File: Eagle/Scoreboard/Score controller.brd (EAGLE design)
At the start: 69.8 x 40.6 mm, 21 parts, among them IC3 74HC595N, Q1 BC338-40, Q2 BC338-40, Q3 BC338-40, Q4 BC338-40, Q5 BC338-40, Q6 BC338-40, Q7 BC338-40

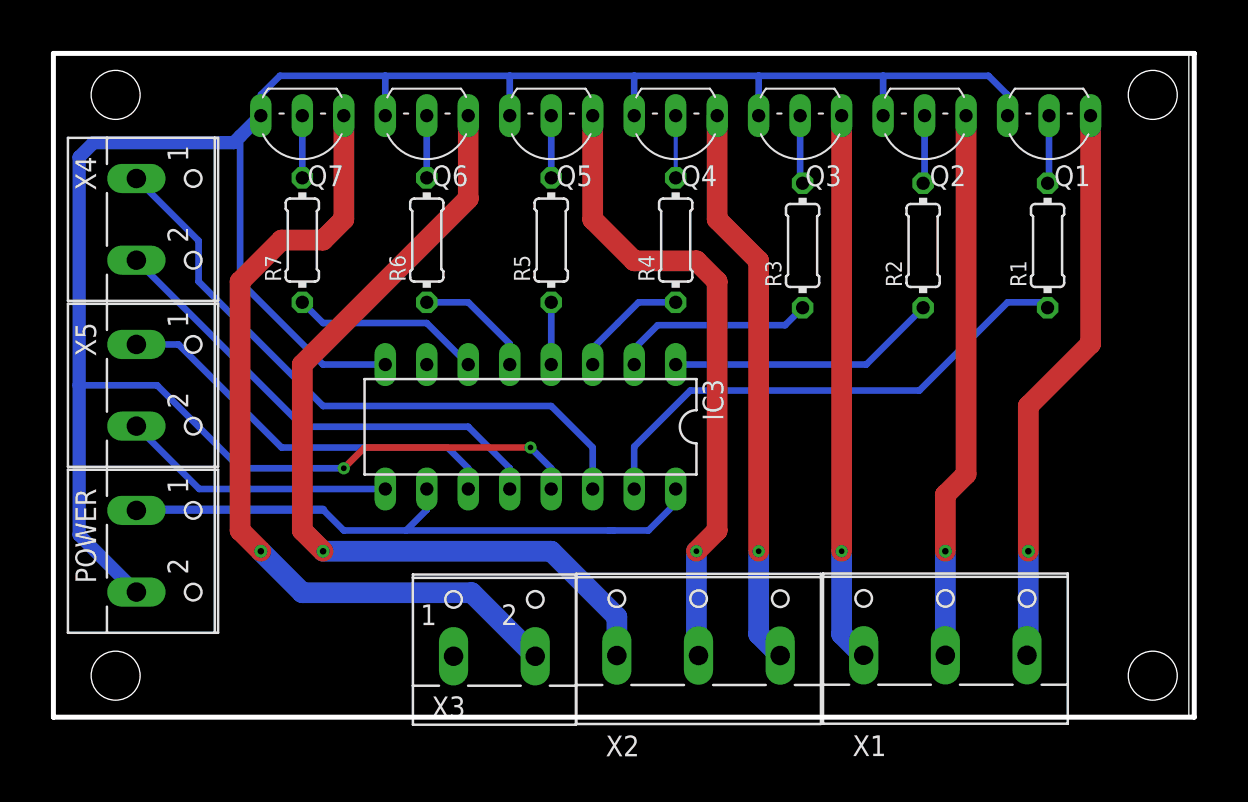
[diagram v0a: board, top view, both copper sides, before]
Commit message: Added polygons
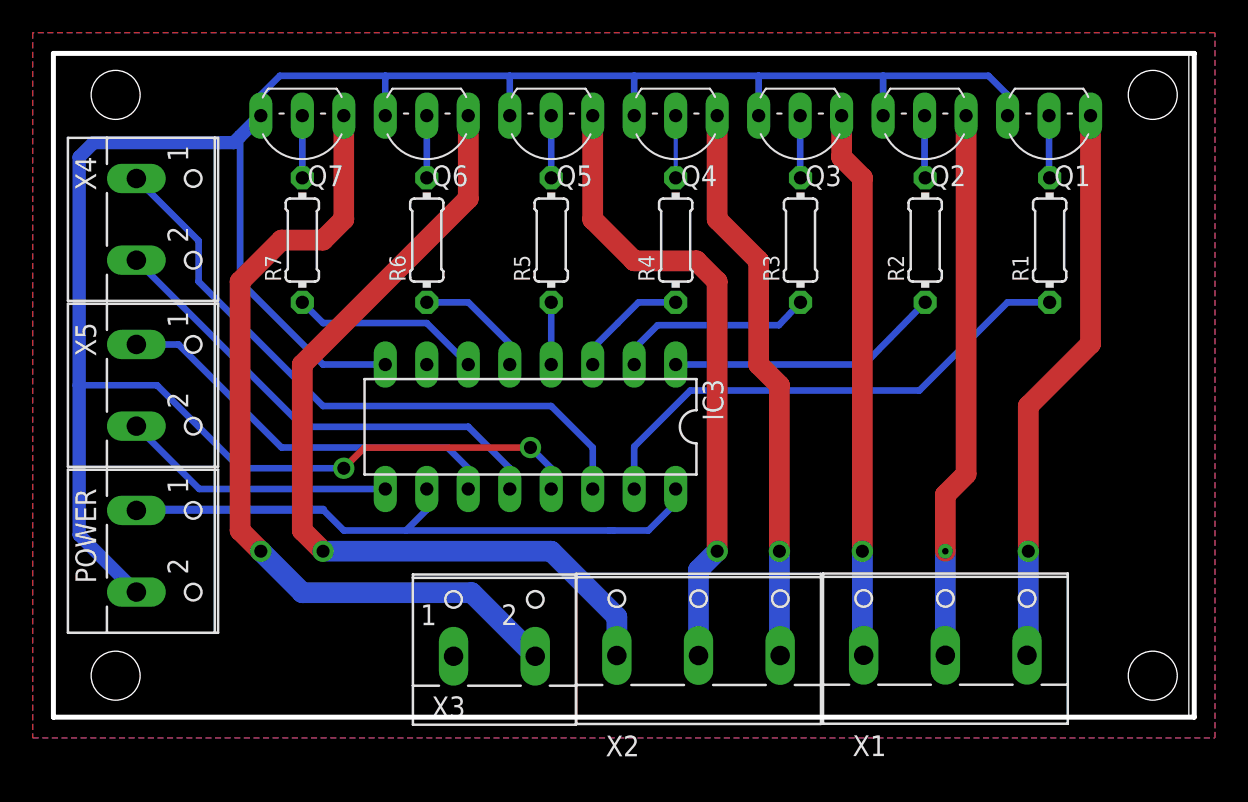
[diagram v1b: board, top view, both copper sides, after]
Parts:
- moved R1 0.35 mm to (61.0, 29.2)
- moved R2 0.35 mm to (53.4, 29.2)
- moved R3 0.35 mm to (45.7, 29.2)
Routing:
- added copper zone on layer 1, net GND
- added copper zone on layer 16, net GND
